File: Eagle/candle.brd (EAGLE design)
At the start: 43.2 x 43.2 mm, 17 parts, among them J1 AVR_SPI_PRG_6NS, U1 Tiny85-20-SMT

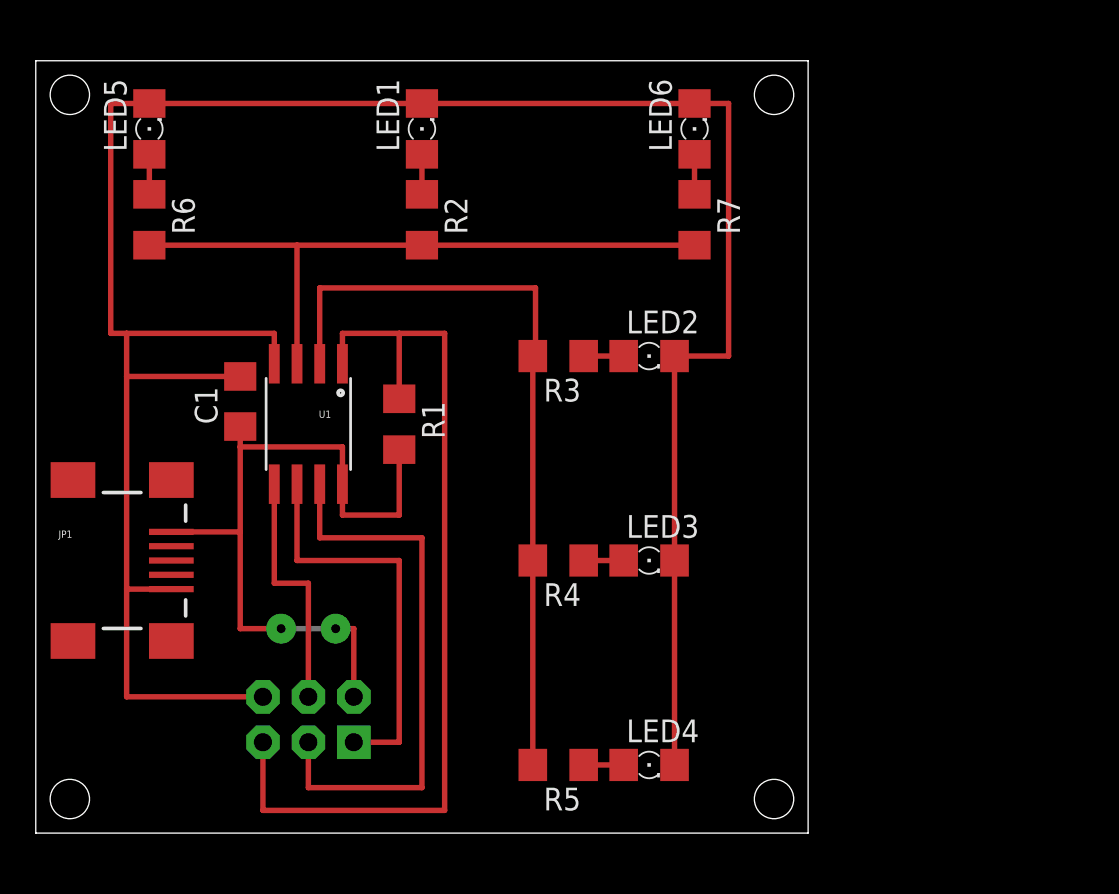
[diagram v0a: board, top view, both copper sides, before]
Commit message: Combine branches into one branch.
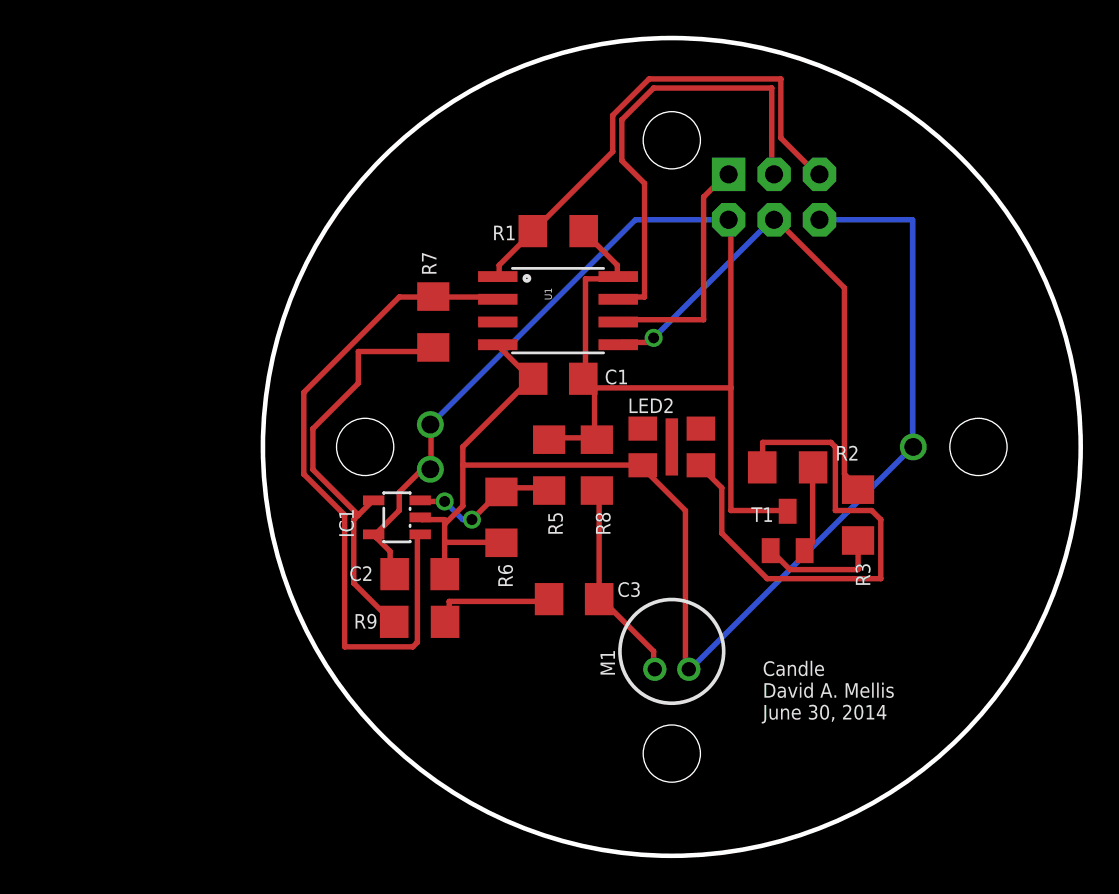
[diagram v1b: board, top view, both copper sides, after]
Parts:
- removed JP1: USB_MINIB, fab:USB_MINIB
- removed LED1, LED3, LED4, LED5, LED6: (no value), led:1206
- removed R4: 330, rcl:R1206
- added C2: 0.1uF, rcl:C1206
- added C3: 1uF, rcl:C1206
- added IC1: AD8615AUJZ, analog-devices:SOT23-5
- added M1: ELECTRETTH, LED Light:ELECTRET_6MM_TH
- added R8: 10K, rcl:R1206
- added R9: 1K, rcl:R1206
- added T1: (no value), transistor:SOT23-BEC
- added U$1: BATTERY-CR2032, LED Light:CR2032_TH
- LED2: value (none) -> ML-EFAB; device led:1206 -> LED Light:ML-E-FAB
- R2: value 330 -> 24
- R3: value 330 -> 1K
- R5, R6, R7: value 330 -> 10K
- moved J1 39.1 mm to (41.3, 35.6), turned to 180 degrees
- moved R6 25.8 mm to (26.0, 17.7), turned to 90 degrees
- moved R2 24.7 mm to (42.0, 20.4), turned to 0 degrees
- moved R3 19.0 mm to (46.0, 17.8), turned to 270 degrees
- moved C1 17.8 mm to (29.2, 25.4), turned to 180 degrees
- moved R5 16.8 mm to (28.7, 20.6), turned to 90 degrees
- moved R7 15.7 mm to (22.2, 28.6)
- moved U1 15.3 mm to (29.2, 29.2), turned to 270 degrees
- moved R1 14.0 mm to (29.2, 33.7), turned to 0 degrees
- moved LED2 5.24 mm to (35.6, 21.6)
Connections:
- removed net N$5: LED6.A, R7.1
- removed net N$7: LED3.A, R4.1
- removed net N$8: LED4.A, R5.1
- new net IN+: IC1.3, R5.1, R6.2
- new net IN-: IC1.4, R7.2, R9.1
- new net MIC: IC1.1, R7.1, U1.2
- net GND: now also C2.2, IC1.2, LED2.C@1, M1.2, R6.1, U$1.-; no longer JP1.GND, LED1.C, LED2.C, LED3.C, LED4.C, LED5.C, LED6.C
- net MOSI: now also R3.1
- net N$1: now also T1.E; no longer R6.2, R7.2, U1.3
- net N$2: now also T1.B; no longer R4.2, R5.2, U1.2
- net N$3: now also LED2.A@1; no longer LED1.A
- net N$4: now also C3.2, M1.1, R8.1; no longer LED2.A, R3.1
- net N$6: now also C3.1, R9.2; no longer LED5.A, R6.1
- net VCC: now also C2.1, IC1.5, R5.2, R8.2, T1.C, U$1.+, U$1.+'; no longer JP1.VBUS
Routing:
- net GND: track 135.0 -> 78.8 mm
- net MIC: track 0.00 -> 38.5 mm
- net N$2: track 43.1 -> 6.95 mm
- net VCC: track 41.7 -> 77.5 mm, vias 2 -> 0
- net N$1: track 37.1 -> 4.84 mm
- net N$3: track 2.24 -> 29.4 mm
- net IN-: track 0.00 -> 23.8 mm
- net RESET: track 51.7 -> 28.2 mm
- net MOSI: track 13.8 -> 28.8 mm, vias 0 -> 1
- net N$4: track 2.24 -> 11.4 mm
- net MISO: track 22.7 -> 13.6 mm
- net IN+: track 0.00 -> 8.57 mm, vias 0 -> 2
- net SCK: track 31.6 -> 26.0 mm
- net N$6: track 2.24 -> 6.89 mm
- net N$8: track 2.24 -> 0.00 mm
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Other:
- board size 43.2 x 43.2 mm -> 45.7 x 45.7 mm
- board text added: "Candle David A. Mellis June 30, 2014"
